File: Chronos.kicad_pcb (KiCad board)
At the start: 2 copper layers, 0 parts

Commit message: Initialize the PCB with outline
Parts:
- added REF**: 60_Outline, local_lib:60_Outline, F.Cu at (154.8, 88.1)
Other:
- board outline added: 285 x 94.6 mm
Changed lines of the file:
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@@
     (tracks 0)
     (zones 0)
-    (modules 0)
+    (modules 1)
     (nets 1)
   )
@@
     (pad_to_mask_clearance 0.2)
     (aux_axis_origin 0 0)
-    (visible_elements FFFFFF7F)
+    (visible_elements 7FFFFFFF)
     (pcbplotparams
       (layerselection 0x00030_80000001)
@@
     (uvia_drill 0.1)
   )
+  (module local_lib:60_Outline locked (layer F.Cu)
+    (at 154.78125 88.10625)
+    (fp_text reference REF** (at -139 50.5) (layer Edge.Cuts) hide
+      (effects (font (size 1 1) (thickness 0.15)))
+    )
+    (fp_text value 60_Outline (at -139 49) (layer F.Fab) hide
+      (effects (font (size 1 1) (thickness 0.15)))
+    )
+    (fp_line (start 138.7 6.54905) (end 142.5 6.54905) (layer F.Mask) (width 2.5019))
+    (fp_line (start 138.7 6.54905) (end 142.5 6.54905) (layer B.Mask) (width 2.5019))
+    (fp_arc (start 138.7 9.2) (end 138.7 6.54905) (angle -90) (layer B.Mask) (width 2.5019))
+    (fp_arc (start 138.7 9.2) (end 138.7 6.54905) (angle -90) (layer F.Mask) (width 2.5019))
+    (fp_arc (start 138.7 9.2) (end 136.04905 9.2) (angle -90) (layer B.Mask) (width 2.5019))
+    (fp_arc (start 138.7 9.2) (end 136.04905 9.2) (angle -90) (layer F.Mask) (width 2.5019))
+    (fp_line (start 138.7 11.85095) (end 142.55 11.85095) (layer F.Mask) (width 2.5019))
+    (fp_line (start 138.7 11.85095) (end 142.55 11.85095) (layer B.Mask) (width 2.5019))
+    (fp_line (start -142.5 6.54905) (end -138.7 6.54905) (layer B.Mask) (width 2.5019))
+    (fp_line (start -142.5 6.54905) (end -138.7 6.54905) (layer F.Mask) (width 2.5019))
+    (fp_arc (start -138.7 9.2) (end -138.7 6.54905) (angle 90) (layer B.Mask) (width 2.5019))
+    (fp_arc (start -138.7 9.2) (end -138.7 6.54905) (angle 90) (layer F.Mask) (width 2.5019))
+    (fp_arc (start -138.7 9.2) (end -136.04905 9.2) (angle 90) (layer F.Mask) (width 2.5019))
+    (fp_arc (start -138.7 9.2) (end -136.04905 9.2) (angle 90) (layer B.Mask) (width 2.5019))
+    (fp_line (start -142.5 11.85095) (end -138.7 11.85095) (layer B.Mask) (width 2.5019))
+    (fp_line (start -142.5 11.85095) (end -138.7 11.85095) (layer F.Mask) (width 2.5019))
+    (fp_line (start 138.7 11.85095) (end 142.55 11.85095) (layer B.Cu) (width 2.5019))
+    (fp_line (start 138.7 6.54905) (end 142.5 6.54905) (layer F.Cu) (width 2.5019))
+    (fp_arc (start 138.7 9.2) (end 136.04905 9.2) (angle -90) (layer F.Cu) (width 2.5019))
+    (fp_arc (start 138.7 9.2) (end 138.7 6.54905) (angle -90) (layer F.Cu) (width 2.5019))
+    (fp_line (start 138.7 6.54905) (end 142.5 6.54905) (layer B.Cu) (width 2.5019))
+    (fp_line (start 138.7 11.85095) (end 142.55 11.85095) (layer F.Cu) (width 2.5019))
+    (fp_arc (start 138.7 9.2) (end 136.04905 9.2) (angle -90) (layer B.Cu) (width 2.5019))
+    (fp_arc (start 138.7 9.2) (end 138.7 6.54905) (angle -90) (layer B.Cu) (width 2.5019))
+    (fp_arc (start -138.7 9.2) (end -138.7 6.54905) (angle 90) (layer B.Cu) (width 2.5019))
+    (fp_arc (start -138.7 9.2) (end -136.04905 9.2) (angle 90) (layer B.Cu) (width 2.5019))
+    (fp_line (start -142.5 11.85095) (end -138.7 11.85095) (layer F.Cu) (width 2.5019))
+    (fp_line (start -142.5 11.85095) (end -138.7 11.85095) (layer B.Cu) (width 2.5019))
+    (fp_arc (start -138.7 9.2) (end -138.7 6.54905) (angle 90) (layer F.Cu) (width 2.5019))
+    (fp_arc (start -138.7 9.2) (end -136.04905 9.2) (angle 90) (layer F.Cu) (width 2.5019))
+    (fp_arc (start -138.7 9.2) (end -137.3 9.2) (angle 90) (layer Edge.Cuts) (width 0.3))
+    (fp_line (start -142.5 6.54905) (end -138.7 6.54905) (layer B.Cu) (width 2.5019))
+    (fp_line (start -142.5 6.54905) (end -138.7 6.54905) (layer F.Cu) (width 2.5019))
+    (fp_line (start 138.7 7.8) (end 142.5 7.8) (layer Edge.Cuts) (width 0.3))
+    (fp_line (start 138.7 10.6) (end 142.5 10.6) (layer Edge.Cuts) (width 0.3))
+    (fp_line (start 142.5 7.8) (end 142.5 -45.3) (layer Edge.Cuts) (width 0.3))
+    (fp_line (start 142.5 10.6) (end 142.5 45.3) (layer Edge.Cuts) (width 0.3))
+    (fp_arc (start 138.7 9.2) (end 137.3 9.2) (angle -90) (layer Edge.Cuts) (width 0.3))
+    (fp_arc (start 138.7 9.2) (end 138.7 7.8) (angle -90) (layer Edge.Cuts) (width 0.3))
+    (fp_line (start -142.5 7.8) (end -142.5 -45.3) (layer Edge.Cuts) (width 0.3))
+    (fp_line (start -138.7 7.8) (end -142.5 7.8) (layer Edge.Cuts) (width 0.3))
+    (fp_arc (start -138.7 9.2) (end -138.7 7.8) (angle 90) (layer Edge.Cuts) (width 0.3))
+    (fp_line (start -142.5 10.6) (end -138.7 10.6) (layer Edge.Cuts) (width 0.3))
+    (fp_line (start -142.5 45.3) (end -142.5 10.6) (layer Edge.Cuts) (width 0.3))
+    (fp_arc (start 140.5 -45.3) (end 140.5 -47.3) (angle 90) (layer Edge.Cuts) (width 0.3))
+    (fp_arc (start 140.5 45.3) (end 142.5 45.3) (angle 90) (layer Edge.Cuts) (width 0.3))
+    (fp_arc (start -140.5 45.3) (end -140.5 47.3) (angle 90) (layer Edge.Cuts) (width 0.3))
+    (fp_arc (start -140.5 -45.3) (end -142.5 -45.3) (angle 90) (layer Edge.Cuts) (width 0.3))
+    (fp_line (start 140.5 -47.3) (end -140.5 -47.3) (layer Edge.Cuts) (width 0.3))
+    (fp_line (start -140.5 47.3) (end 140.5 47.3) (layer Edge.Cuts) (width 0.3))
+    (pad 1 thru_hole circle (at -117.3 -19.4) (size 7.0013 7.0013) (drill 2.4994) (layers *.Cu *.Mask))
+    (pad 1 thru_hole circle (at -14.3 -0.3) (size 7.00024 7.00024) (drill oval 5.00126 2.49936) (layers *.Cu *.Mask))
+    (pad 1 thru_hole circle (at 48 37.9) (size 7.00024 7.00024) (drill oval 5.00126 2.49936) (layers *.Cu *.Mask))
+    (pad 1 thru_hole circle (at 117.55 -19.4) (size 7.00024 7.00024) (drill oval 5.00126 2.49936) (layers *.Cu *.Mask))
+  )
 )

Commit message: Adjust PCB design page size
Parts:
- moved REF** 23.9 mm to (177.7, 81.3)
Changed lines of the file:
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@@
     (nets 1)
   )
-  (page A4)
+  (page A3)
   (layers
     (0 F.Cu signal)
@@
   )
   (module local_lib:60_Outline locked (layer F.Cu)
-    (at 154.78125 88.10625)
+    (at 177.725 81.3125)
     (fp_text reference REF** (at -139 50.5) (layer Edge.Cuts) hide
       (effects (font (size 1 1) (thickness 0.15)))

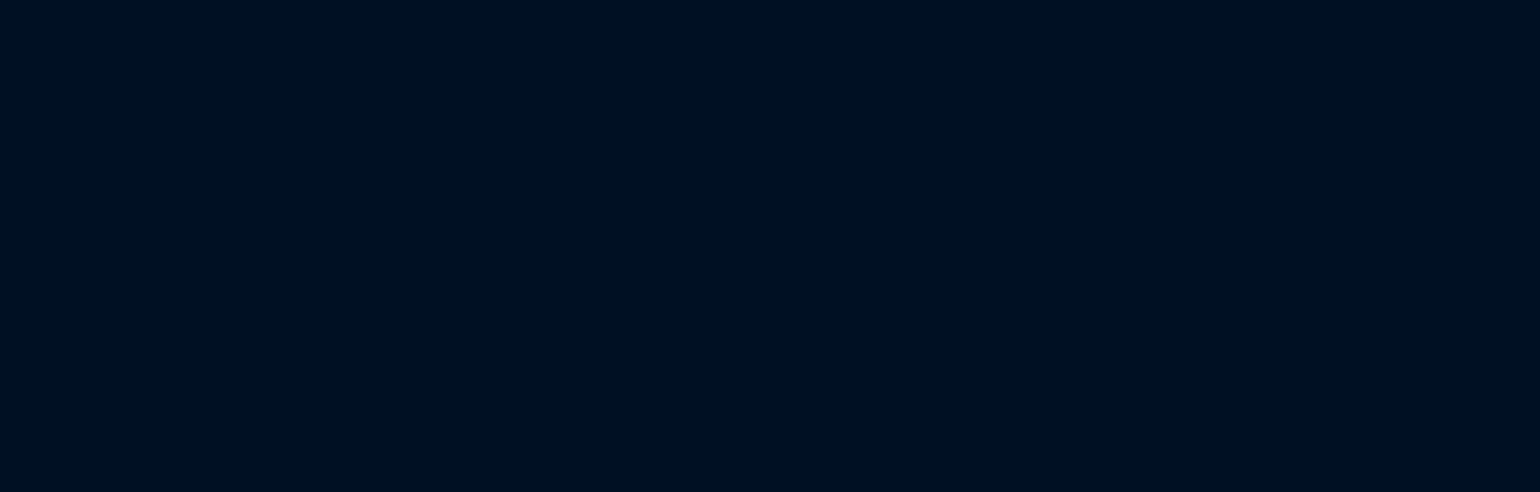
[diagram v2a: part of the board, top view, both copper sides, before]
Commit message: Import netlist
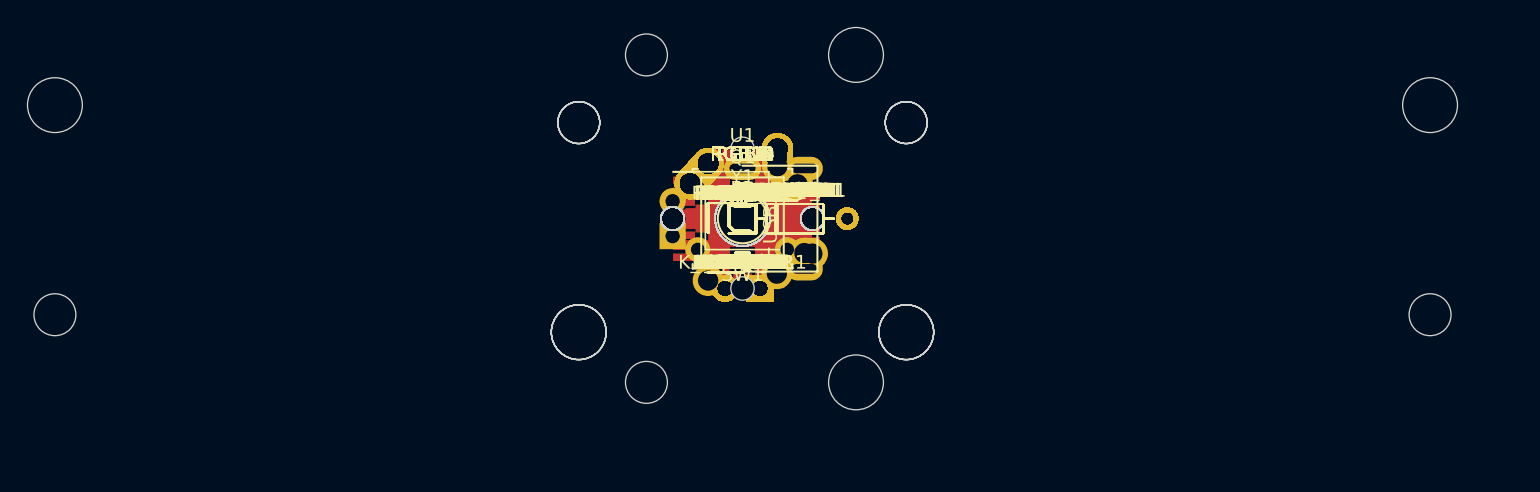
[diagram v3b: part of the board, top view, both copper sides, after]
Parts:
- added C1, C2: 22p, Capacitors_SMD:C_0805_HandSoldering, F.Cu at (0.00, 0.00)
- added C3: 1uF, Capacitors_SMD:C_0805_HandSoldering, F.Cu at (0.00, 0.00)
- added C4, C5, CR1, CR10, CR11, CR12, CR13, CR14, CR2, CR3, CR4, CR5, CR6, CR7, CR8, CR9: 0.1u, Capacitors_SMD:C_0805_HandSoldering, F.Cu at (0.00, 0.00)
- added C6: 4.7u, Capacitors_SMD:C_0805_HandSoldering, F.Cu at (0.00, 0.00)
- added D_#0_1, D_#1, D_#2, D_#3, D_#4, D_#5, D_#6, D_#7, D_#8, D_#9, D_'1, D_,1, D_-1, D_.1, D_/1, D_;1, D_=1, D_A1, D_ALT1, D_B1, D_BACK1, D_C1, D_CAPS1, D_CTRL1, D_D1, D_DEL1, D_DOWN1, D_E1, D_ENTER1, D_ESC1, D_F1, D_FN1, D_G1, D_H1, D_I1, D_ISO\1, D_ISO`1, D_J1, D_K1, D_L1, D_LEFT1, D_M1, D_N1, D_O1, D_P1, D_Q1, D_R1, D_RIGHT1, D_RSHIFT1, D_S1, D_SHIFT1, D_SPACE1, D_T1, D_TAB1, D_U1, D_UP1, D_V1, D_W1, D_WIN1, D_X1, D_Y1, D_Z1, D_[1, D_\1, D_]1, D_`1: 1N4148, Diodes_THT:D_DO-35_SOD27_P7.62mm_Horizontal, F.Cu at (0.00, 0.00)
- added F1: 500mA, Fuse_Holders_and_Fuses:Fuse_SMD1206_HandSoldering, F.Cu at (0.00, 0.00)
- added K_#0_1, K_#1, K_#2, K_#3, K_#4, K_#5, K_#6, K_#7, K_#8, K_#9, K_'1, K_,1, K_-1, K_.1, K_/2, K_;1, K_=1, K_A1, K_B1, K_BACK1, K_C1, K_D1, K_DEL1, K_DOWN1, K_E1, K_ESC1, K_F1, K_FN1, K_G1, K_H1, K_I1, K_ISO\1, K_ISO`1, K_J1, K_K1, K_L1, K_LEFT1, K_M1, K_N1, K_O1, K_P1, K_Q1, K_R1, K_RIGHT1, K_RSHIFT1, K_S1, K_T1, K_U1, K_UP1, K_V1, K_W1, K_X1, K_Y1, K_Z1, K_[1, K_]1, K_`1: MX-1U, MX_Alps_Hybrid:MX-1U, F.Cu at (0.00, 0.00)
- added K_/1, K_CAPS1: MX-1.75U, MX_Alps_Hybrid:MX-1.75U, F.Cu at (0.00, 0.00)
- added K_ALT1, K_ALT2, K_CTRL1, K_FN2, K_MENU1, K_RALT1, K_RCTRL1, K_RWIN1, K_WIN1: MX-1.25U, MX_Alps_Hybrid:MX-1.25U, F.Cu at (0.00, 0.00)
- added K_BACK2: MX-2U, MX_Alps_Hybrid:MX-2U, F.Cu at (0.00, 0.00)
- added K_CMD1, K_CTRL2, K_RCMD1, K_RCTRL2, K_TAB1, K_\1: MX-1.5U, MX_Alps_Hybrid:MX-1.5U, F.Cu at (0.00, 0.00)
- added K_ENTER1, K_SHIFT1: MX-2.25U, MX_Alps_Hybrid:MX-2.25U, F.Cu at (0.00, 0.00)
- added K_ISOENTER1: MX-ISO, MX_Alps_Hybrid:MX-ISO-Combined, F.Cu at (0.00, 0.00)
- added K_RSHIFT2: MX-2.75U, MX_Alps_Hybrid:MX-2.75U, F.Cu at (0.00, 0.00)
- added K_SPACE1: MX-6.25U-FLIPPED, MX_Alps_Hybrid:MX-6.25U-ReversedStabilizers, F.Cu at (0.00, 0.00)
- added K_SPACE2: MX-6.5U, MX_Alps_Hybrid:MX-6.5U, F.Cu at (0.00, 0.00)
- added Q1: NSS40301MZ4T1G, TO_SOT_Packages_SMD:SOT-223-3_TabPin2, F.Cu at (0.00, 0.00)
- added R1, R5: 10k, Resistors_SMD:R_0805_HandSoldering, F.Cu at (0.00, 0.00)
- added R2, R3: 22, Resistors_SMD:R_0805_HandSoldering, F.Cu at (0.00, 0.00)
- added R4: 1.5k, Resistors_SMD:R_0805_HandSoldering, F.Cu at (0.00, 0.00)
- added RGB1, RGB10, RGB11, RGB12, RGB13, RGB14, RGB2, RGB3, RGB4, RGB5, RGB6, RGB7, RGB8, RGB9: WS2812B, WS2812B:WS2812B, F.Cu at (0.00, 0.00)
- added R_#0_1, R_#1, R_#2, R_#3, R_#4, R_#5, R_#6, R_#7, R_#8, R_#9, R_'1, R_,1, R_-1, R_.1, R_/1, R_;1, R_=1, R_A1, R_ALT1, R_B1, R_BACK1, R_C1, R_CAPS1, R_CTRL1, R_D1, R_DEL1, R_DOWN1, R_E1, R_ENTER1, R_ESC1, R_F1, R_FN1, R_G1, R_H1, R_I1, R_ISO\1, R_ISO`1, R_J1, R_K1, R_L1, R_LEFT1, R_M1, R_N1, R_O1, R_P1, R_Q1, R_R1, R_RIGHT1, R_RSHIFT1, R_S1, R_SHIFT1, R_SPACE1, R_T1, R_TAB1, R_U1, R_UP1, R_V1, R_W1, R_WIN1, R_X1, R_Y1, R_Z1, R_[1, R_\1, R_]1, R_`1: 2.7k, Resistors_SMD:R_1206_HandSoldering, F.Cu at (0.00, 0.00)
- added SW1: SW_PUSH, Molex-0548190589:PushButton_6x6mm_TH, F.Cu at (0.00, 0.00)
- added U1: ATMEGA32U2-AU, Housings_QFP:TQFP-32_7x7mm_Pitch0.8mm, F.Cu at (0.00, 0.00)
- added USB1: Molex-0548190589, Molex-0548190589:Molex-0548190589, F.Cu at (0.00, 0.00)
- added Y1: 16MHz, Crystals:Crystal_SMD_3225-4pin_3.2x2.5mm_HandSoldering, F.Cu at (0.00, 0.00)

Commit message: Begin construction of basic layout
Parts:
- moved REF** 144.1 mm to (209.6, -59.2)
- moved K_#3 120.7 mm to (111.9, 45.2)
- moved K_#2 103.3 mm to (92.9, 45.2)
- moved K_#1 86.6 mm to (73.8, 45.2)
- moved K_ESC1 71.0 mm to (54.8, 45.2)
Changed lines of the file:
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@@
   )
   (module local_lib:60_Outline locked (layer F.Cu)
-    (at 177.725 81.3125)
+    (at 209.5625 -59.23125)
     (fp_text reference REF** (at -139 50.5) (layer Edge.Cuts) hide
       (effects (font (size 1 1) (thickness 0.15)))
@@
   )
   (module MX_Alps_Hybrid:MX-1U (layer F.Cu)
-    (at 0 0)
+    (at 73.81875 45.24375)
     (fp_text reference K_#1 (at 0 3.175) (layer F.SilkS)
       (effects (font (size 1 1) (thickness 0.15)))
@@
   )
   (module MX_Alps_Hybrid:MX-1U (layer F.Cu)
-    (at 0 0)
+    (at 92.86875 45.24375)
     (fp_text reference K_#2 (at 0 3.175) (layer F.SilkS)
       (effects (font (size 1 1) (thickness 0.15)))
@@
   )
   (module MX_Alps_Hybrid:MX-1U (layer F.Cu)
-    (at 0 0)
+    (at 111.91875 45.24375)
     (fp_text reference K_#3 (at 0 3.175) (layer F.SilkS)
       (effects (font (size 1 1) (thickness 0.15)))
@@
   )
   (module MX_Alps_Hybrid:MX-1U (layer F.Cu)
-    (at 0 0)
+    (at 54.76875 45.24375)
     (fp_text reference K_ESC1 (at 0 3.175) (layer F.SilkS)
       (effects (font (size 1 1) (thickness 0.15)))

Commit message: Row 1 switch layout of PCB
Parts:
- moved K_BACK1 328.9 mm to (323.9, 57.1)
- moved K_BACK2 319.5 mm to (314.3, 57.1)
- moved K_DEL1 310.1 mm to (304.8, 57.1)
- moved K_=1 291.4 mm to (285.8, 57.1)
- moved K_-1 272.8 mm to (266.7, 57.1)
- moved K_#0_1 254.2 mm to (247.7, 57.1)
- moved K_#9 235.6 mm to (228.6, 57.1)
- moved K_#8 217.2 mm to (209.6, 57.1)
- moved K_#7 198.9 mm to (190.5, 57.1)
- moved K_#6 180.7 mm to (171.4, 57.1)
- moved K_#5 162.8 mm to (152.4, 57.1)
- moved K_#4 145.1 mm to (133.3, 57.1)
- moved K_#1 12.1 mm to (76.2, 57.1)
- moved K_ESC1 12.1 mm to (57.1, 57.1)
- moved K_#2 12.1 mm to (95.2, 57.1)
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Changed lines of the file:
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@@
   (general
     (links 647)
-    (no_connects 178)
-    (area 0 0 0 0)
+    (no_connects 186)
+    (area -62.187501 -106.881251 353.563451 55.043751)
     (thickness 1.6)
     (drawings 0)
@@
   )
   (module MX_Alps_Hybrid:MX-1U (layer F.Cu)
-    (at 0 0)
+    (at 247.65 57.15)
     (fp_text reference K_#0_1 (at 0 3.175) (layer F.SilkS)
       (effects (font (size 1 1) (thickness 0.15)))
@@
   )
   (module MX_Alps_Hybrid:MX-1U (layer F.Cu)
-    (at 73.81875 45.24375)
+    (at 76.2 57.15)
     (fp_text reference K_#1 (at 0 3.175) (layer F.SilkS)
       (effects (font (size 1 1) (thickness 0.15)))
@@
   )
   (module MX_Alps_Hybrid:MX-1U (layer F.Cu)
-    (at 92.86875 45.24375)
+    (at 95.25 57.15)
     (fp_text reference K_#2 (at 0 3.175) (layer F.SilkS)
       (effects (font (size 1 1) (thickness 0.15)))
@@
   )
   (module MX_Alps_Hybrid:MX-1U (layer F.Cu)
-    (at 111.91875 45.24375)
+    (at 114.3 57.15)
     (fp_text reference K_#3 (at 0 3.175) (layer F.SilkS)
       (effects (font (size 1 1) (thickness 0.15)))
@@
   )
   (module MX_Alps_Hybrid:MX-1U (layer F.Cu)
-    (at 0 0)
+    (at 133.35 57.15)
     (fp_text reference K_#4 (at 0 3.175) (layer F.SilkS)
       (effects (font (size 1 1) (thickness 0.15)))
@@
   )
   (module MX_Alps_Hybrid:MX-1U (layer F.Cu)
-    (at 0 0)
+    (at 152.4 57.15)
     (fp_text reference K_#5 (at 0 3.175) (layer F.SilkS)
       (effects (font (size 1 1) (thickness 0.15)))
@@
   )
   (module MX_Alps_Hybrid:MX-1U (layer F.Cu)
-    (at 0 0)
+    (at 171.45 57.15)
     (fp_text reference K_#6 (at 0 3.175) (layer F.SilkS)
       (effects (font (size 1 1) (thickness 0.15)))
@@
   )
   (module MX_Alps_Hybrid:MX-1U (layer F.Cu)
-    (at 0 0)
+    (at 190.5 57.15)
     (fp_text reference K_#7 (at 0 3.175) (layer F.SilkS)
       (effects (font (size 1 1) (thickness 0.15)))
@@
   )
   (module MX_Alps_Hybrid:MX-1U (layer F.Cu)
-    (at 0 0)
+    (at 209.55 57.15)
     (fp_text reference K_#8 (at 0 3.175) (layer F.SilkS)
       (effects (font (size 1 1) (thickness 0.15)))
@@
   )
   (module MX_Alps_Hybrid:MX-1U (layer F.Cu)
-    (at 0 0)
+    (at 228.6 57.15)
     (fp_text reference K_#9 (at 0 3.175) (layer F.SilkS)
       (effects (font (size 1 1) (thickness 0.15)))
@@
   )
   (module MX_Alps_Hybrid:MX-1U (layer F.Cu)
-    (at 0 0)
+    (at 266.7 57.15)
     (fp_text reference K_-1 (at 0 3.175) (layer F.SilkS)
       (effects (font (size 1 1) (thickness 0.15)))
@@
   )
   (module MX_Alps_Hybrid:MX-1U (layer F.Cu)
-    (at 0 0)
+    (at 285.75 57.15)
     (fp_text reference K_=1 (at 0 3.175) (layer F.SilkS)
       (effects (font (size 1 1) (thickness 0.15)))
@@
   )
   (module MX_Alps_Hybrid:MX-1U (layer F.Cu)
-    (at 0 0)
+    (at 323.85 57.15)
     (fp_text reference K_BACK1 (at 0 3.175) (layer F.SilkS)
       (effects (font (size 1 1) (thickness 0.15)))
@@
   )
   (module MX_Alps_Hybrid:MX-2U (layer F.Cu)
-    (at 0 0)
+    (at 314.325 57.15)
     (fp_text reference K_BACK2 (at 0 3.175) (layer F.SilkS)
       (effects (font (size 1 1) (thickness 0.15)))
@@
   )
   (module MX_Alps_Hybrid:MX-1U (layer F.Cu)
-    (at 0 0)
+    (at 304.8 57.15)
     (fp_text reference K_DEL1 (at 0 3.175) (layer F.SilkS)
       (effects (font (size 1 1) (thickness 0.15)))
@@
   )
   (module MX_Alps_Hybrid:MX-1U (layer F.Cu)
-    (at 54.76875 45.24375)
+    (at 57.15 57.15)
     (fp_text reference K_ESC1 (at 0 3.175) (layer F.SilkS)
       (effects (font (size 1 1) (thickness 0.15)))
